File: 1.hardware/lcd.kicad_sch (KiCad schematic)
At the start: 0 parts

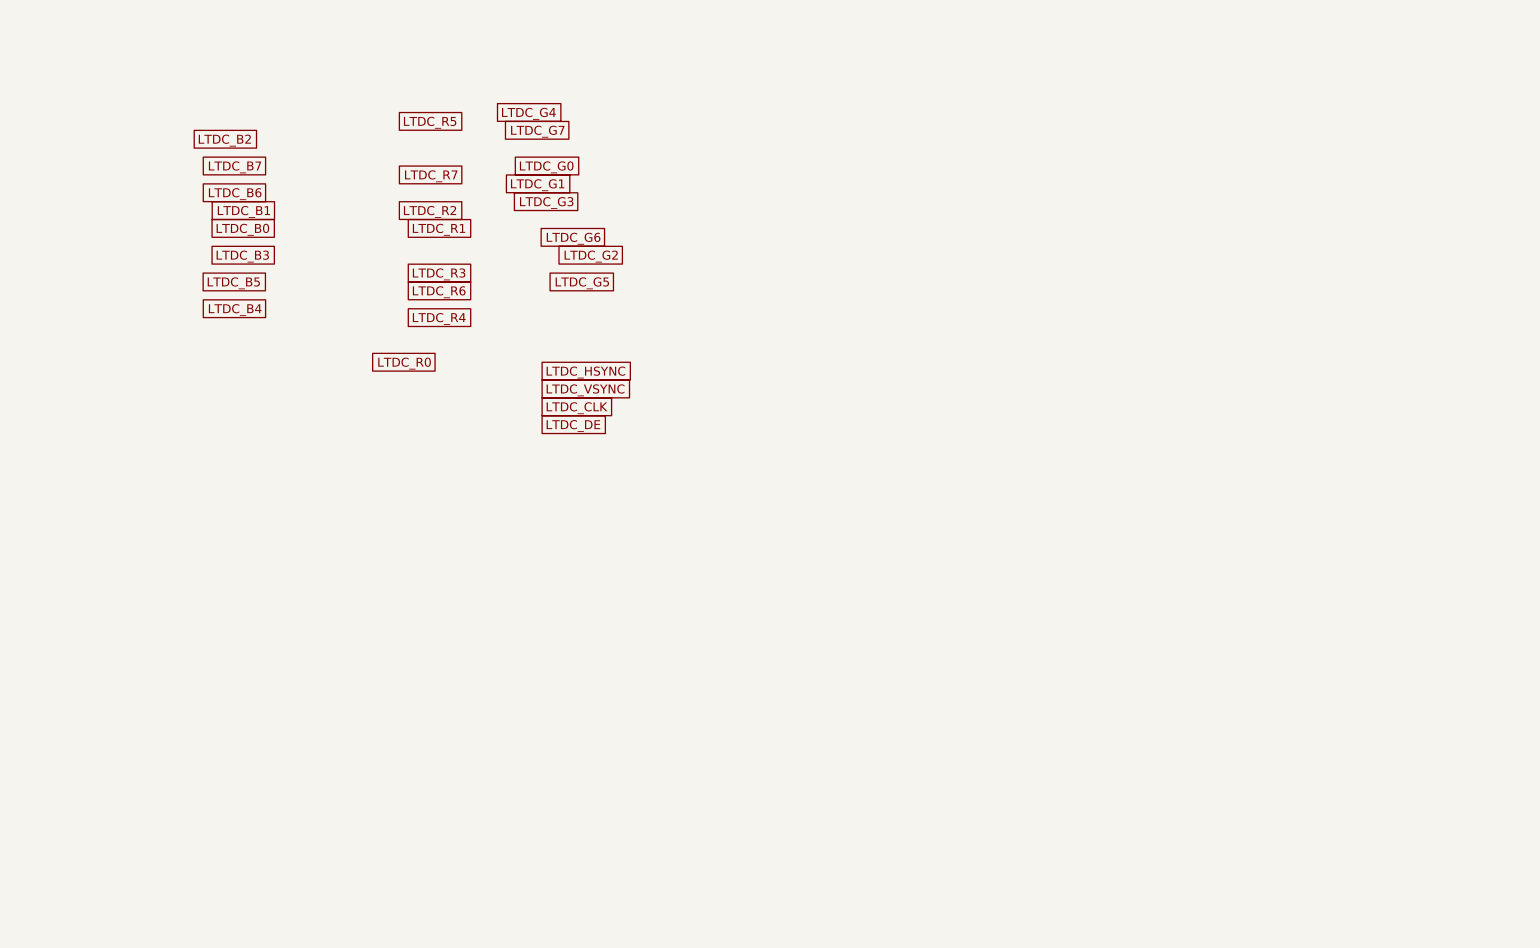
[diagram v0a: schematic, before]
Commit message: 중간 저장
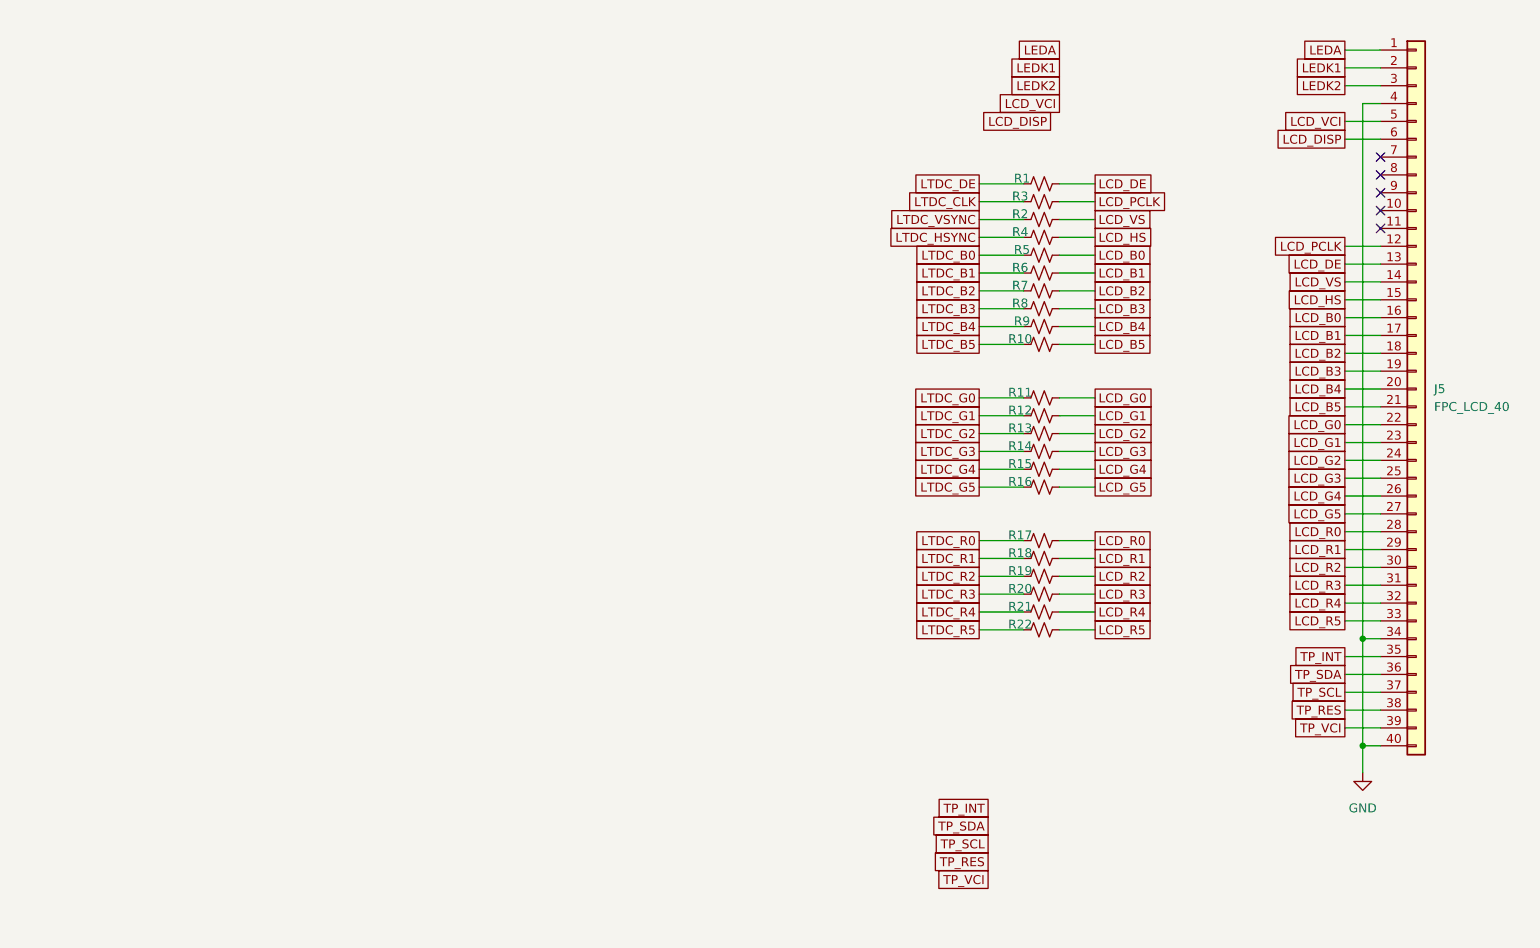
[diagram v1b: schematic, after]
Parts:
- added J5: FPC_LCD_40, symbol Connector_Generic:Conn_01x40
- added R1, R10, R11, R12, R13, R14, R15, R16, R17, R18, R19, R2, R20, R21, R22, R3, R4, R5, R6, R7, R8, R9: 22R/0.063w, symbol Device:R_Small_US
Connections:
- net LTDC_B0: now also R5.1
- net LTDC_B1: now also R6.1
- net LTDC_B2: now also R7.1
- net LTDC_B3: now also R8.1
- net LTDC_B4: now also R9.1
- net LTDC_B5: now also R10.1
- net LTDC_CLK: now also R3.1
- net LTDC_DE: now also R1.1
- net LTDC_G0: now also R11.1
- net LTDC_G1: now also R12.1
- net LTDC_G2: now also R13.1
- net LTDC_G3: now also R14.1
- net LTDC_G4: now also R15.1
- net LTDC_G5: now also R16.1
- net LTDC_HSYNC: now also R4.1
- net LTDC_R0: now also R17.1
- net LTDC_R1: now also R18.1
- net LTDC_R2: now also R19.1
- net LTDC_R3: now also R20.1
- net LTDC_R4: now also R21.1
- net LTDC_R5: now also R22.1
- net LTDC_VSYNC: now also R2.1
- new net GND: J5.34 (Pin_34), J5.4 (Pin_4), J5.40 (Pin_40)
- new net LCD_B0: J5.16 (Pin_16), R5.2
- new net LCD_B1: J5.17 (Pin_17), R6.2
- new net LCD_B2: J5.18 (Pin_18), R7.2
- new net LCD_B3: J5.19 (Pin_19), R8.2
- new net LCD_B4: J5.20 (Pin_20), R9.2
- new net LCD_B5: J5.21 (Pin_21), R10.2
- new net LCD_DE: J5.13 (Pin_13), R1.2
- new net LCD_DISP: J5.6 (Pin_6)
- new net LCD_G0: J5.22 (Pin_22), R11.2
- new net LCD_G1: J5.23 (Pin_23), R12.2
- new net LCD_G2: J5.24 (Pin_24), R13.2
- new net LCD_G3: J5.25 (Pin_25), R14.2
- new net LCD_G4: J5.26 (Pin_26), R15.2
- new net LCD_G5: J5.27 (Pin_27), R16.2
- new net LCD_HS: J5.15 (Pin_15), R4.2
- new net LCD_PCLK: J5.12 (Pin_12), R3.2
- new net LCD_R0: J5.28 (Pin_28), R17.2
- new net LCD_R1: J5.29 (Pin_29), R18.2
- new net LCD_R2: J5.30 (Pin_30), R19.2
- new net LCD_R3: J5.31 (Pin_31), R20.2
- new net LCD_R4: J5.32 (Pin_32), R21.2
- new net LCD_R5: J5.33 (Pin_33), R22.2
- new net LCD_VCI: J5.5 (Pin_5)
- new net LCD_VS: J5.14 (Pin_14), R2.2
- new net LEDA: J5.1 (Pin_1)
- new net LEDK1: J5.2 (Pin_2)
- new net LEDK2: J5.3 (Pin_3)
- new net TP_INT: J5.35 (Pin_35)
- new net TP_RES: J5.38 (Pin_38)
- new net TP_SCL: J5.37 (Pin_37)
- new net TP_SDA: J5.36 (Pin_36)
- new net TP_VCI: J5.39 (Pin_39)
- no-connect marks 0 -> 5

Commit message: 중간 저장2
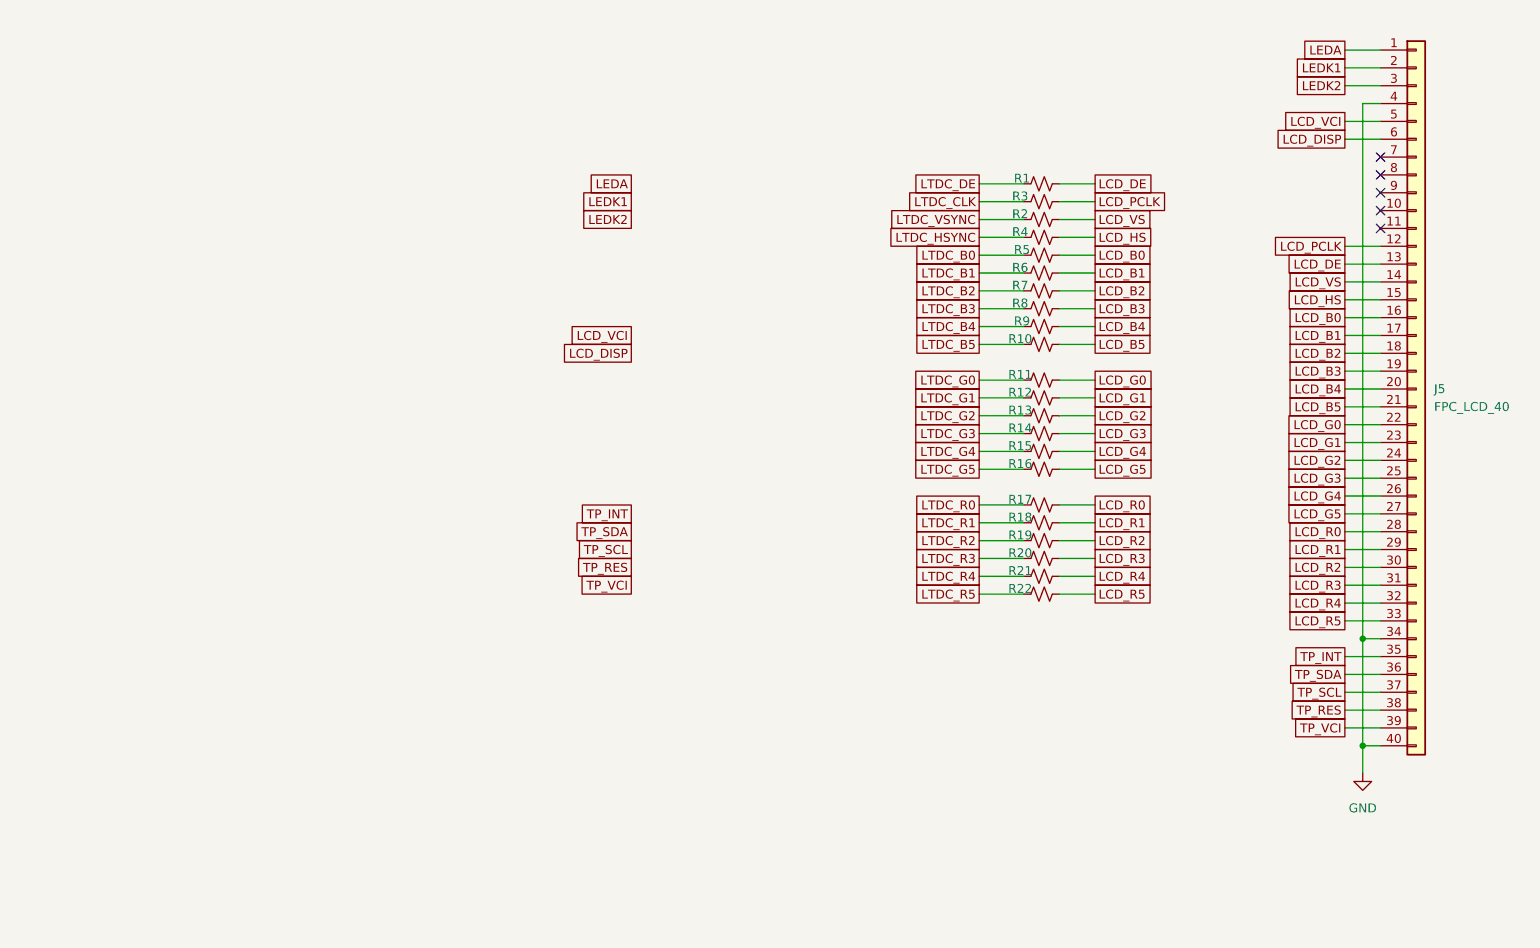
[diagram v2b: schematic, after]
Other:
- moved on the sheet: R11, R12, R13, R14, R15, R16, R17, R18, R19, R20, R21, R22

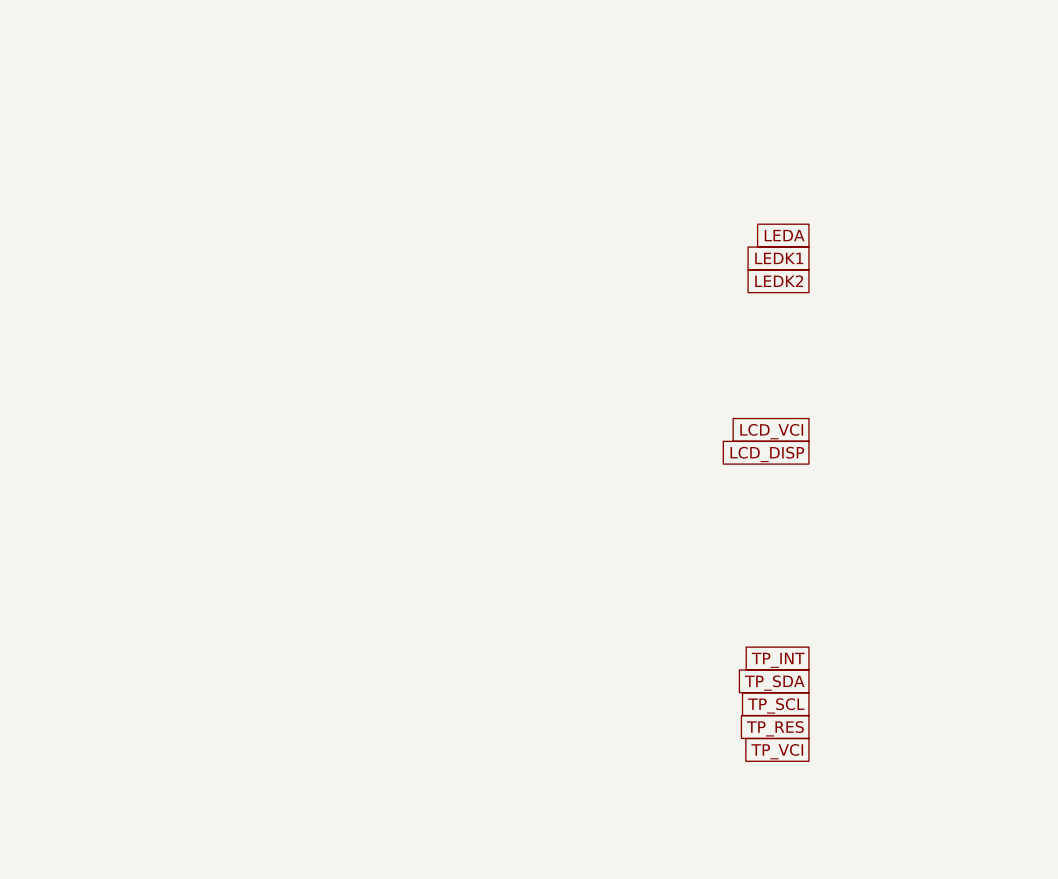
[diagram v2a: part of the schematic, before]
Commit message: 중간저장
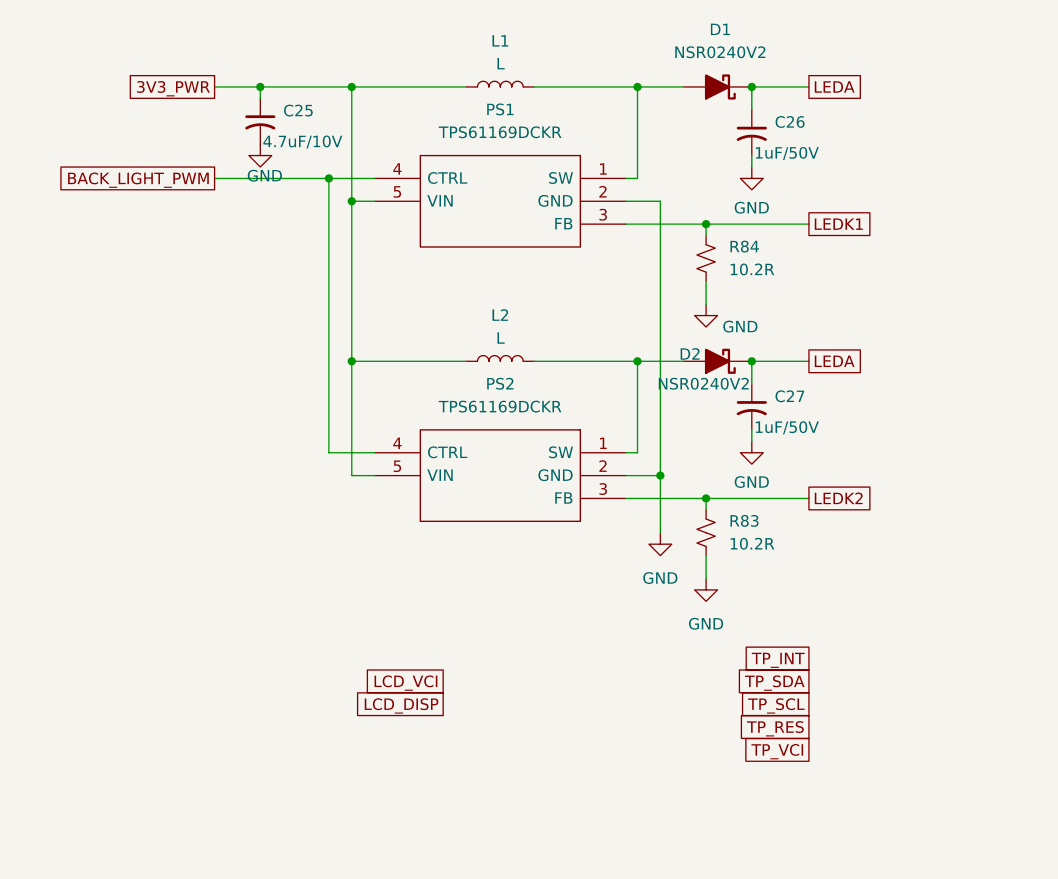
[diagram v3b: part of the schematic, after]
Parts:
- added C25: 4.7uF/10V, Capacitor_SMD:C_0603_1608Metric, symbol Device:C_Small_US
- added C26, C27: 1uF/50V, Capacitor_SMD:C_0603_1608Metric, symbol Device:C_Small_US
- added D1, D2: NSR0240V2, PCM_Diode_SMD_AKL:D_SOD-523, symbol PCM_Diode_Schottky_AKL:NSR0240V2
- added L1, L2: L, symbol Device:L
- added PS1, PS2: TPS61169DCKR, SOT65P210X110-5N, symbol SamacSys_Parts:TPS61169DCKR
- added R83, R84: 10.2R, symbol Device:R_Small_US
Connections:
- net GND: now also C25.2, C26.2, C27.2, PS1.2 (GND), PS2.2 (GND), R83.2, R84.2
- net LEDA: now also C26.1, C27.1, D1.1 (K), D2.1 (K)
- net LEDK1: now also PS1.3 (FB), R84.1
- net LEDK2: now also PS2.3 (FB), R83.1
- new net: D1.2 (A), L1.2, PS1.1 (SW)
- new net: D2.2 (A), L2.2, PS2.1 (SW)
- new net 3V3_PWR: C25.1, L1.1, L2.1, PS1.5 (VIN), PS2.5 (VIN)
- new net BACK_LIGHT_PWM: PS1.4 (CTRL), PS2.4 (CTRL)

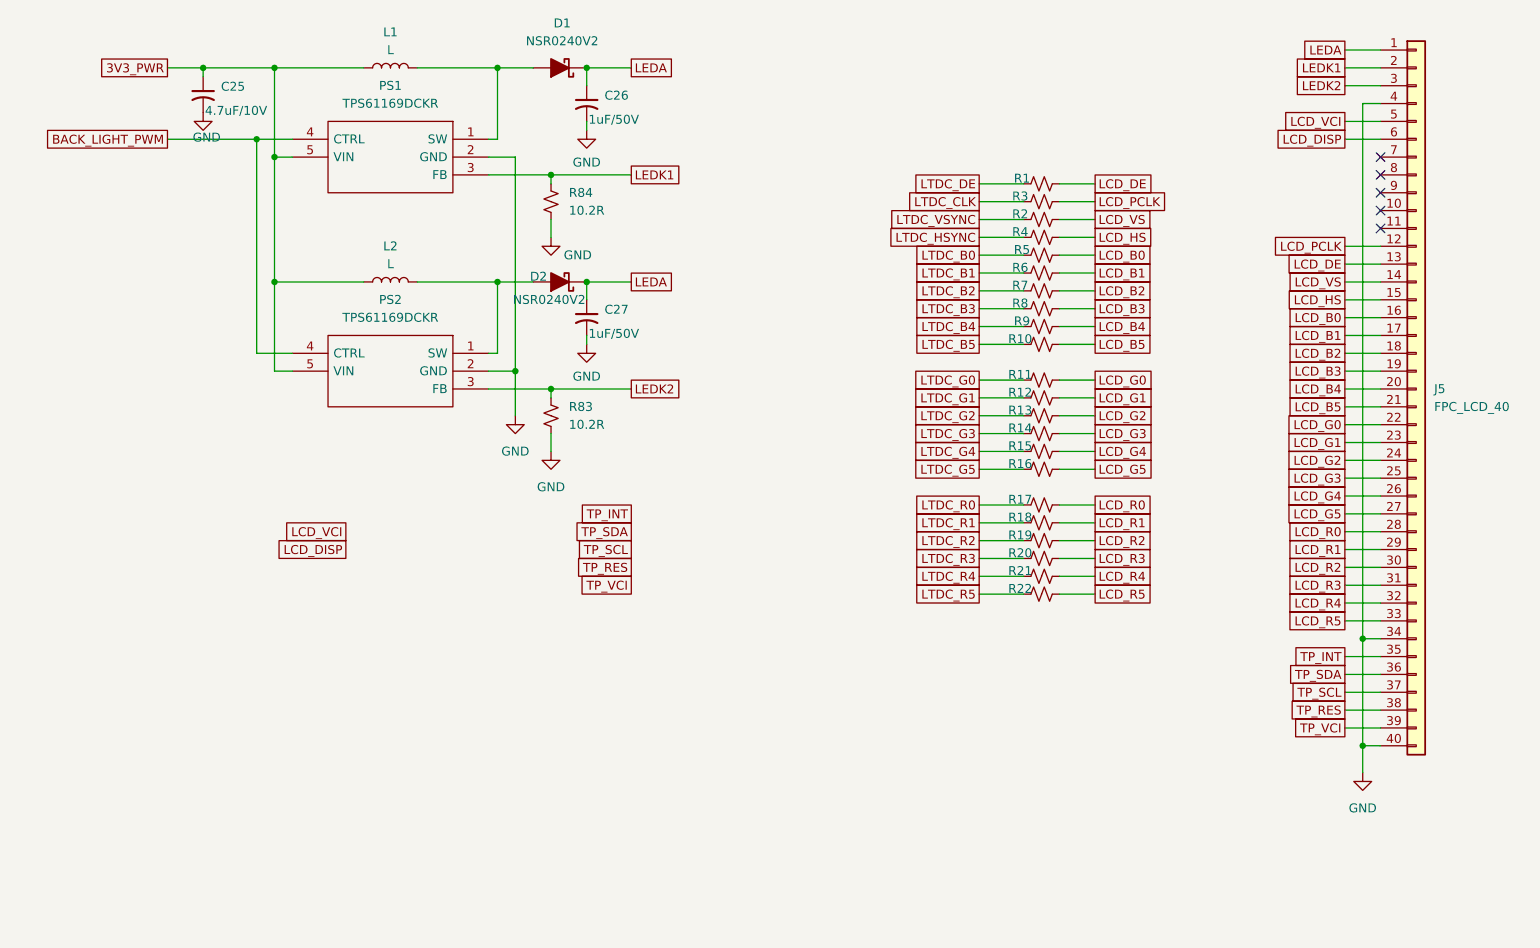
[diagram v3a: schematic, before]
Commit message: 중간 저장
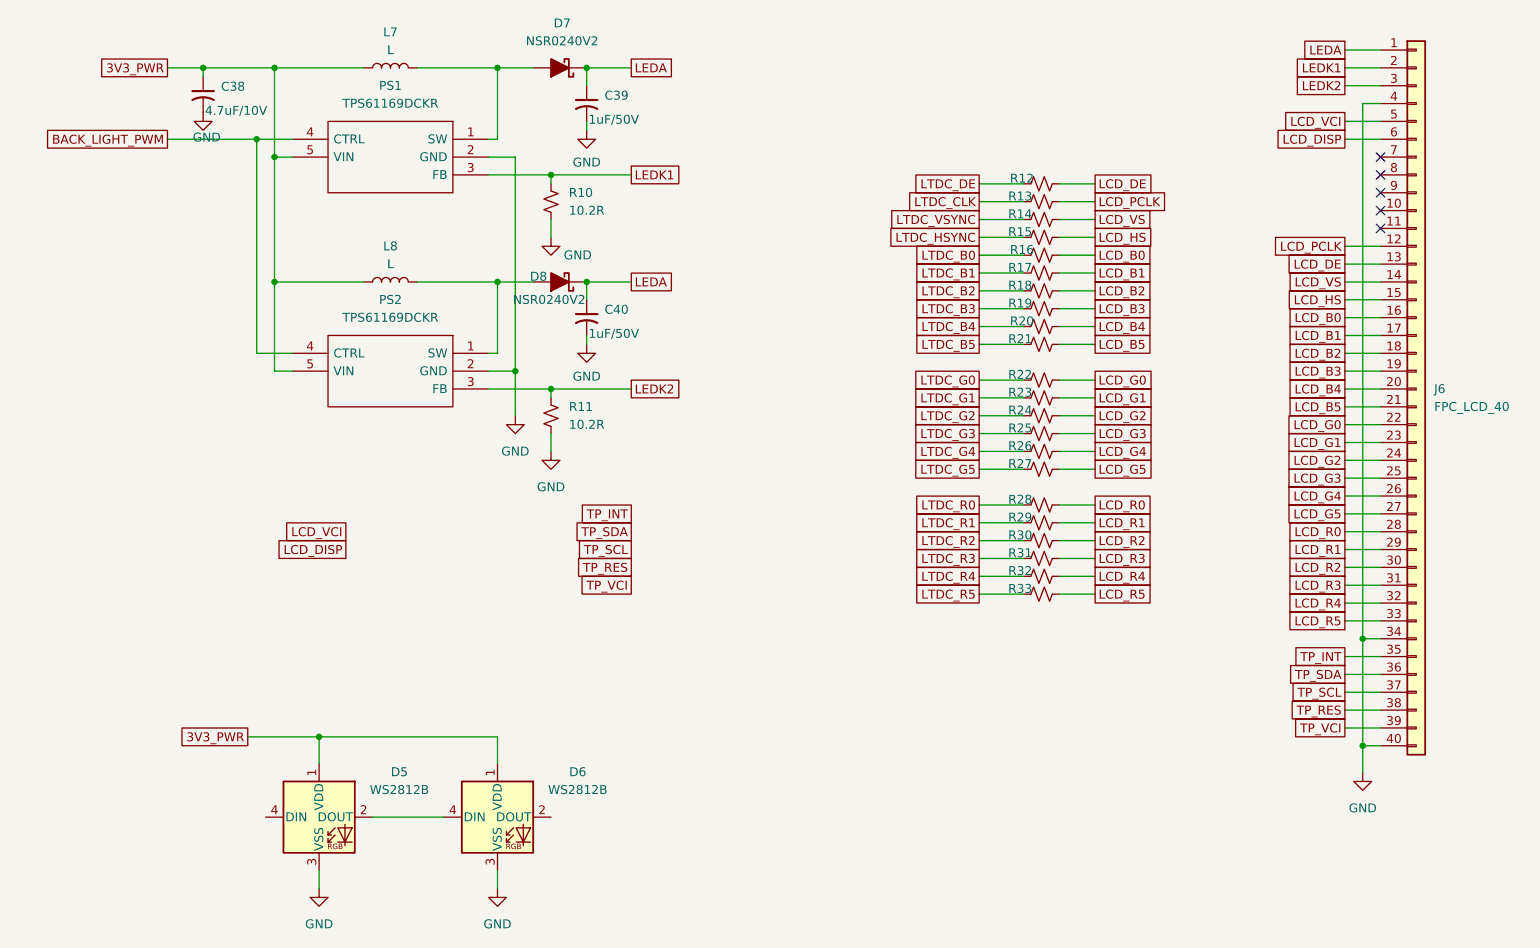
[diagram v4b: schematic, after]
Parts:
- added D5, D6: WS2812B, LED_SMD:LED_WS2812B_PLCC4_5.0x5.0mm_P3.2mm, symbol LED:WS2812B
- renumbered C25 to C38, C26 to C39, C27 to C40, D1 to D7, D2 to D8, J5 to J6, L1 to L7, L2 to L8, R84 to R10, R83 to R11, R1 to R12, R3 to R13, R2 to R14, R4 to R15, R5 to R16, R6 to R17, R7 to R18, R8 to R19, R9 to R20, R10 to R21, R11 to R22, R12 to R23, R13 to R24, R14 to R25, R15 to R26, R16 to R27, R17 to R28, R18 to R29, R19 to R30, R20 to R31, R21 to R32, R22 to R33
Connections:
- net 3V3_PWR: now also D5.1 (VDD), D6.1 (VDD)
- net GND: now also D5.3 (VSS), D6.3 (VSS)
- new net: D5.2 (DOUT), D6.4 (DIN)
